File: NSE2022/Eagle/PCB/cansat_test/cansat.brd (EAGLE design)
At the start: 85 x 100 mm, 80 parts, among them U2 CP2102N-A01-GQFN28

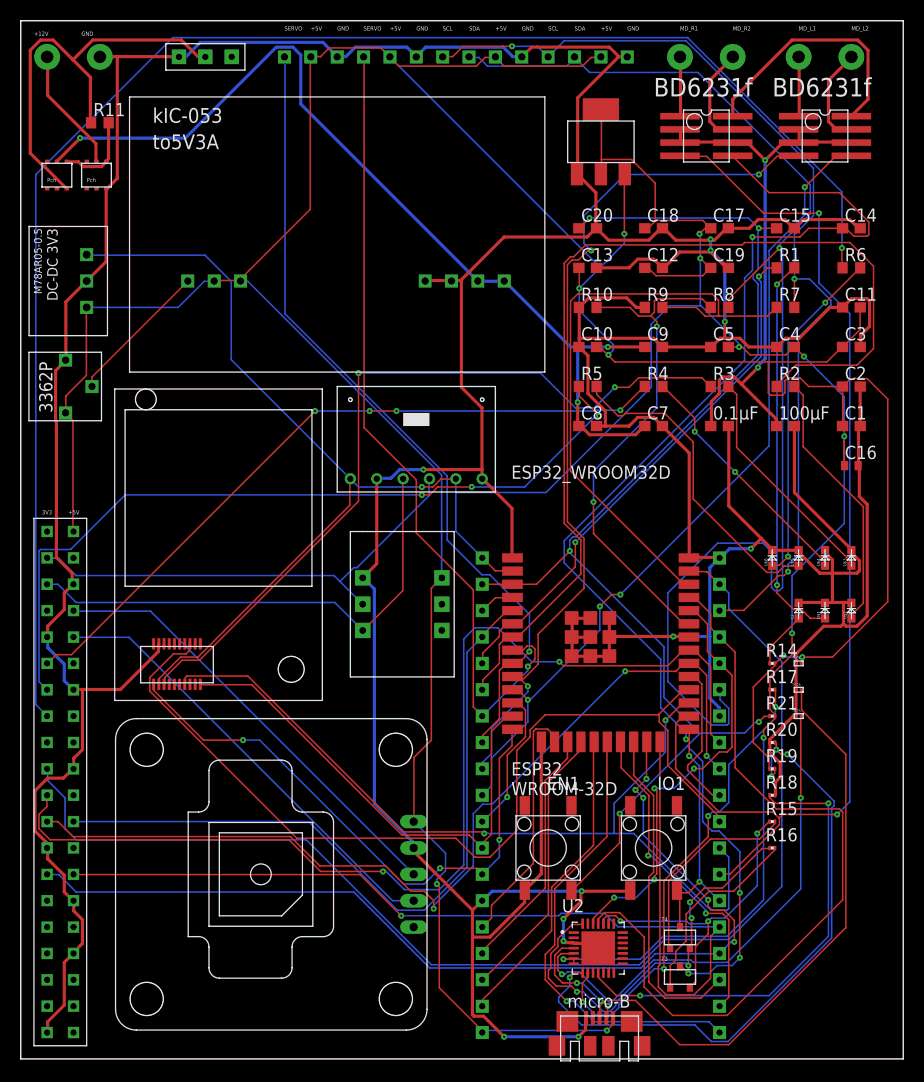
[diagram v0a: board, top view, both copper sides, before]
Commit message: a
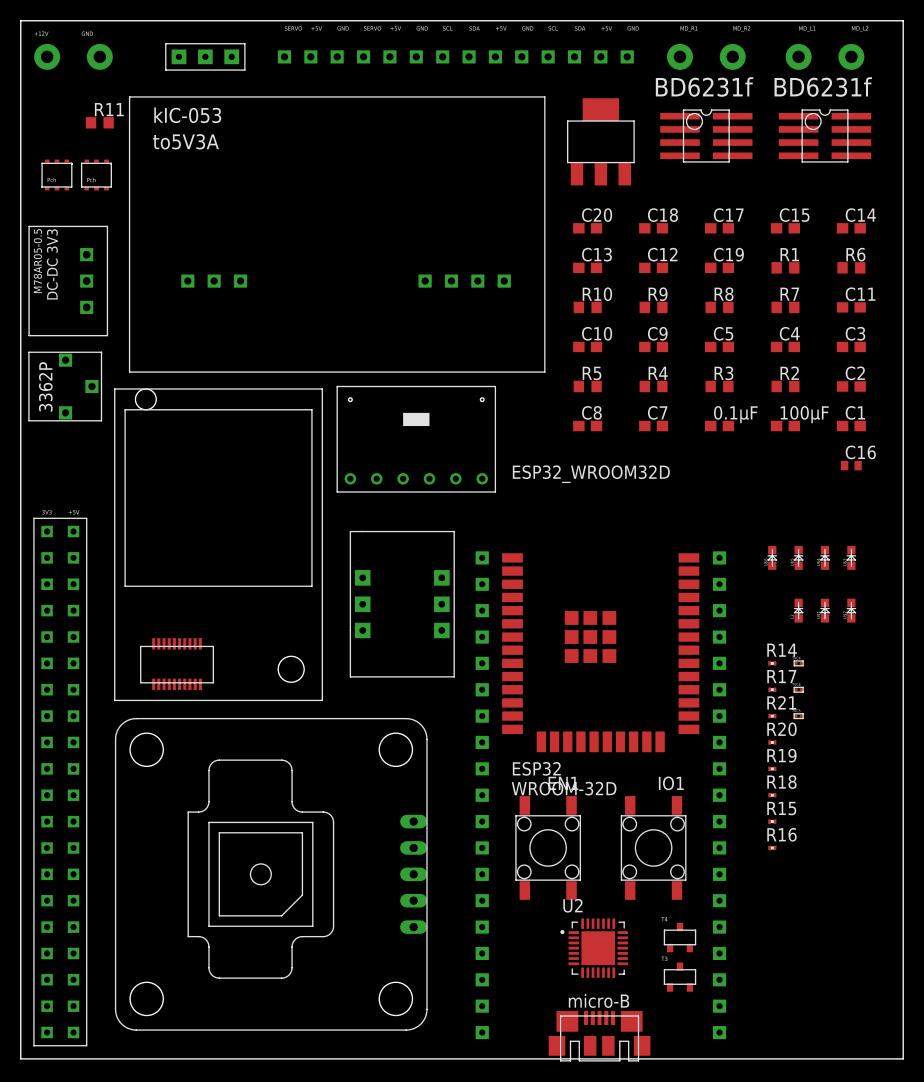
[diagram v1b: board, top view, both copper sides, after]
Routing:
- net GND: track 643.6 -> 0.00 mm, vias 11 -> 0
- net +5V: track 339.7 -> 0.00 mm, vias 7 -> 0
- net +3V3: track 262.0 -> 0.00 mm, vias 9 -> 0
- net LED6: track 149.3 -> 0.00 mm, vias 1 -> 0
- net EN: track 148.9 -> 0.00 mm, vias 8 -> 0
- net AS_SDA: track 123.6 -> 0.00 mm, vias 1 -> 0
- net RP_MOSI: track 119.2 -> 0.00 mm
- net MD_RB: track 114.1 -> 0.00 mm, vias 4 -> 0
- net MD_RF: track 107.3 -> 0.00 mm, vias 2 -> 0
- net RP_MISO: track 104.4 -> 0.00 mm, vias 2 -> 0
- net RP_RX: track 99.5 -> 0.00 mm, vias 1 -> 0
- net AS_SCL: track 96.8 -> 0.00 mm, vias 3 -> 0
- net LED2: track 96.8 -> 0.00 mm
- net RP_TX: track 95.3 -> 0.00 mm, vias 5 -> 0
- net +12V: track 90.6 -> 0.00 mm, vias 3 -> 0
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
